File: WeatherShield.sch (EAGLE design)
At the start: 81 parts, among them Q1 BSS138, Q2 BSS138, U1 DS3231SN, U2 LT3652, U4 MPL3115A2LGA8, U5 HTU21D

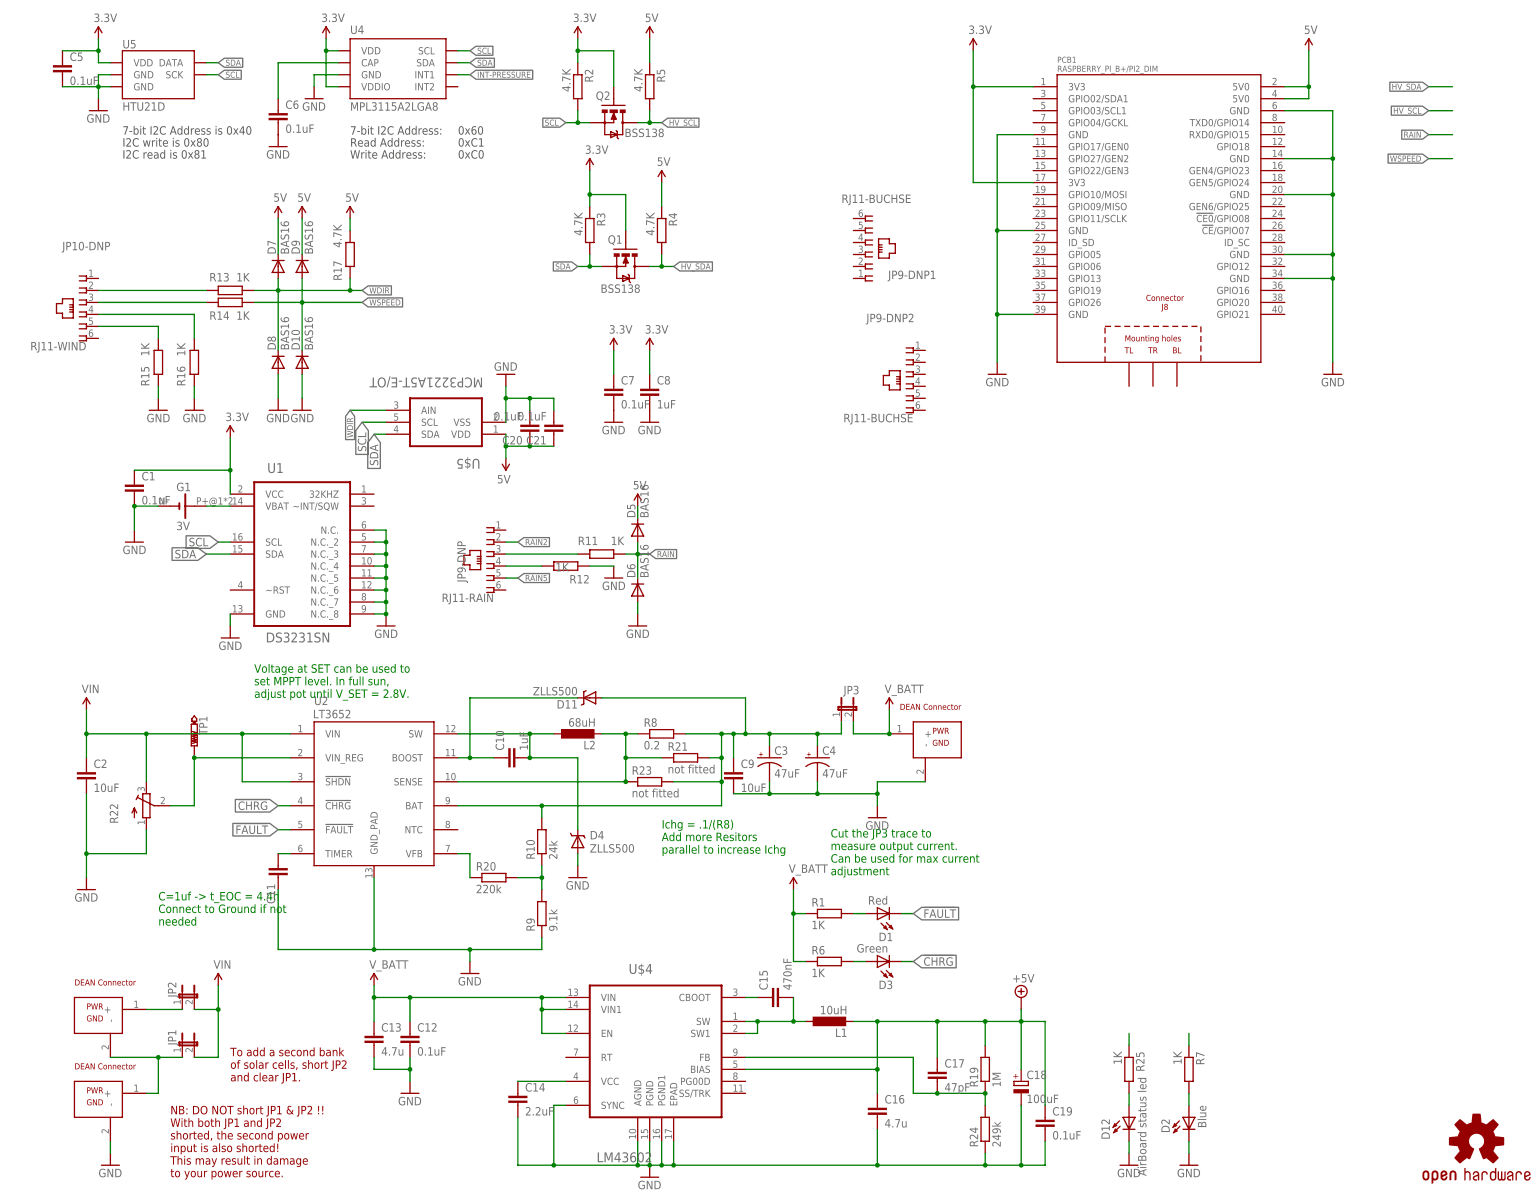
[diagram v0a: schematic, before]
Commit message: Power parts
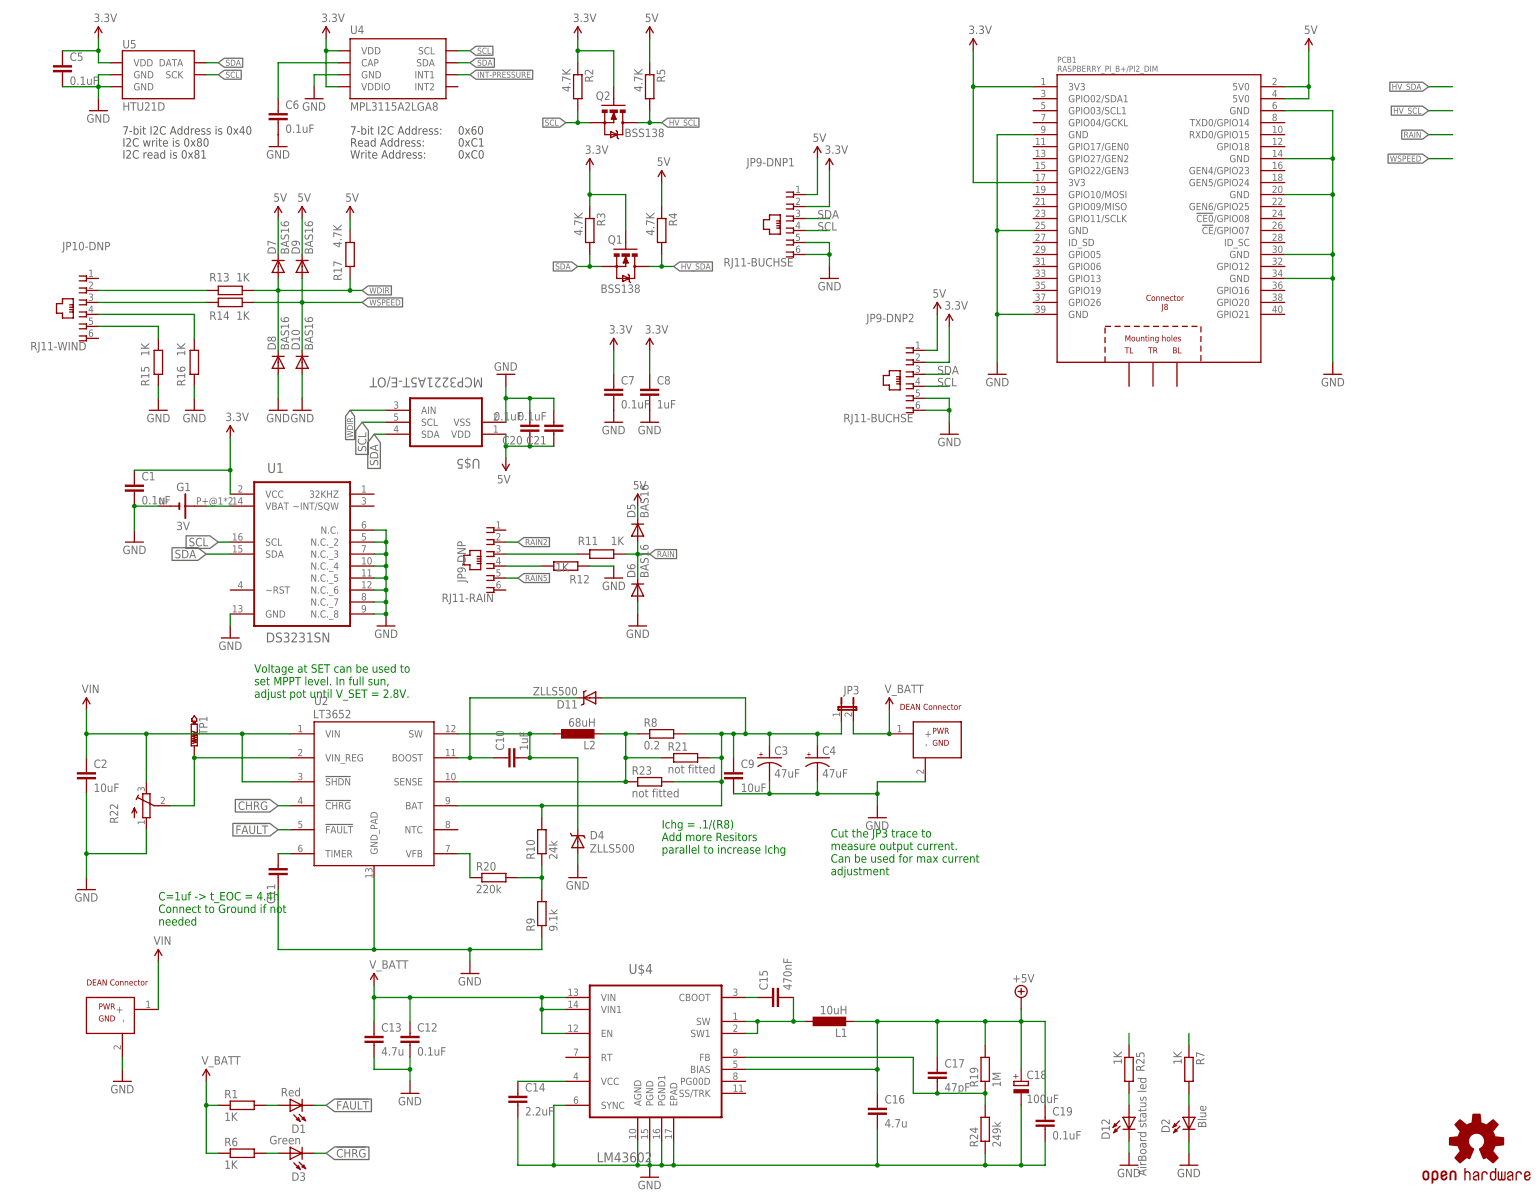
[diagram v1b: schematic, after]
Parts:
- removed JP1, JP2: (no value), jumper:JP1E
- removed U$1: DEAN_CONNECTOR, FSE_Weather_Shield:DEAN_CONNECTOR
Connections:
- removed net N$14: JP1.1, U$1.-, U$2.+
- removed net SFSASDF: JP2.1, U$1.+
- net 5V: now also JP9-DNP1.1, JP9-DNP2.1
- net GND: now also JP9-DNP1.5, JP9-DNP1.6, JP9-DNP2.5, JP9-DNP2.6
- net SCL: now also JP9-DNP1.4, JP9-DNP2.4
- net SDA: now also JP9-DNP1.3, JP9-DNP2.3
- net VCC: now also JP9-DNP1.2, JP9-DNP2.2
- net VIN: now also U$2.+; no longer JP1.2, JP2.2
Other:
- note removed: "NB: DO NOT short JP1 & JP2 !! With both JP1 and JP2 shorted, the second power input is also shorted! This may result in damage to your power source."
- note removed: "To add a second bank of solar cells, short JP2 and clear JP1."
- moved on the sheet: D1, D3, JP9-DNP1, R1, R6
